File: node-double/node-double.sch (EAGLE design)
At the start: 33 parts, among them IC1 TP4056, IC3 24C02, U1 ATMEGA328P_TQFP, U2 3.3V/150mA

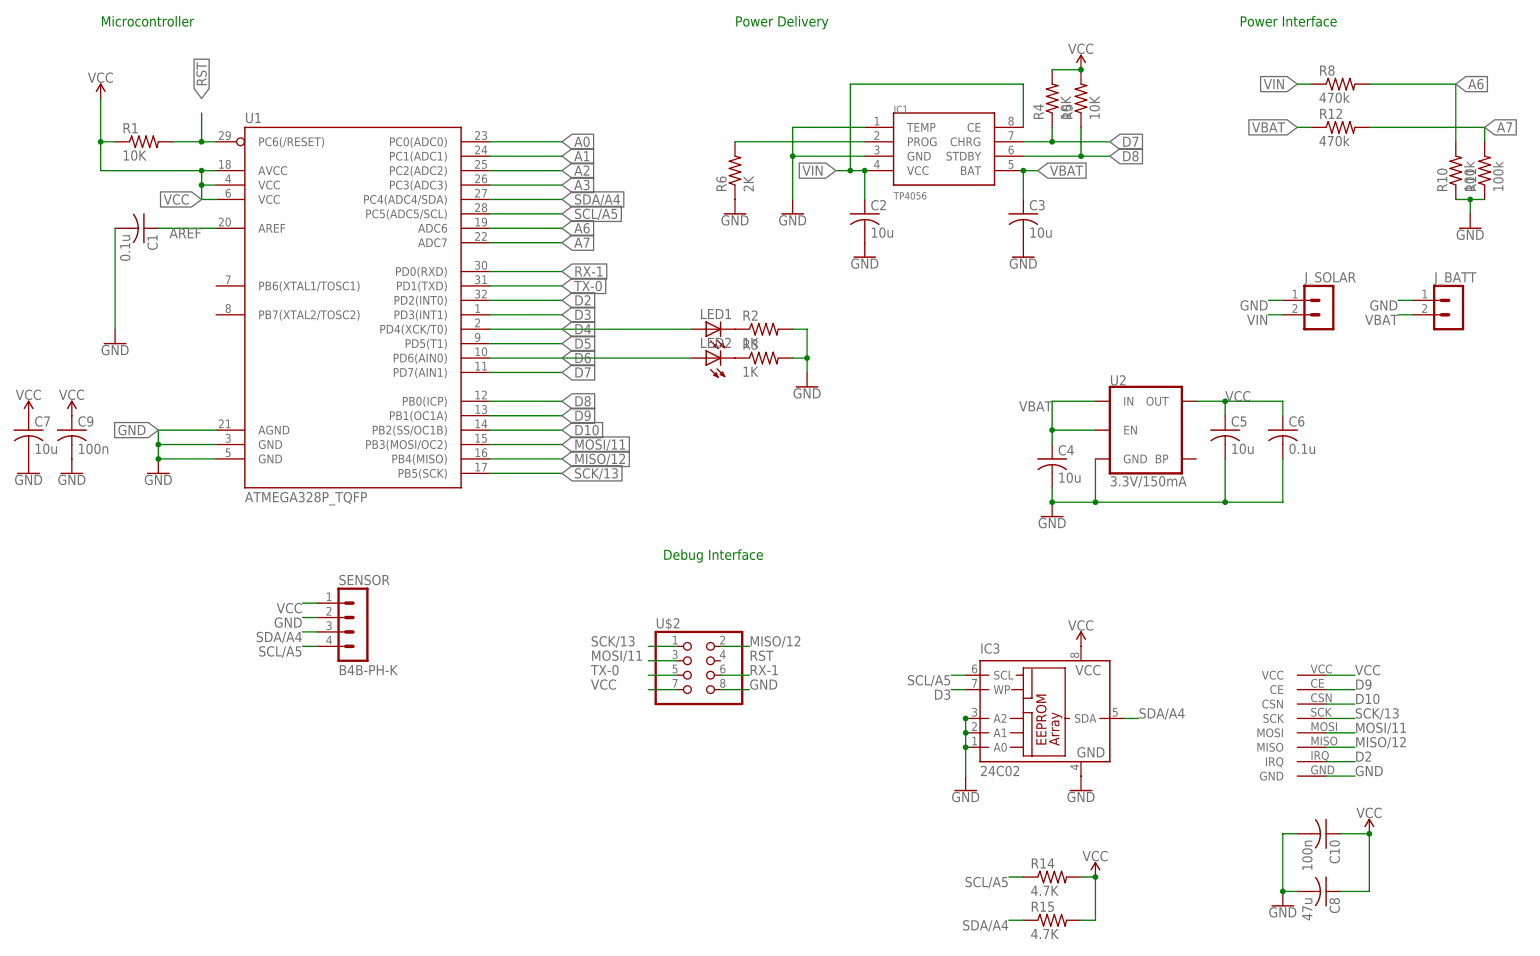
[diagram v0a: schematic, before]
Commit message: Scratch progress
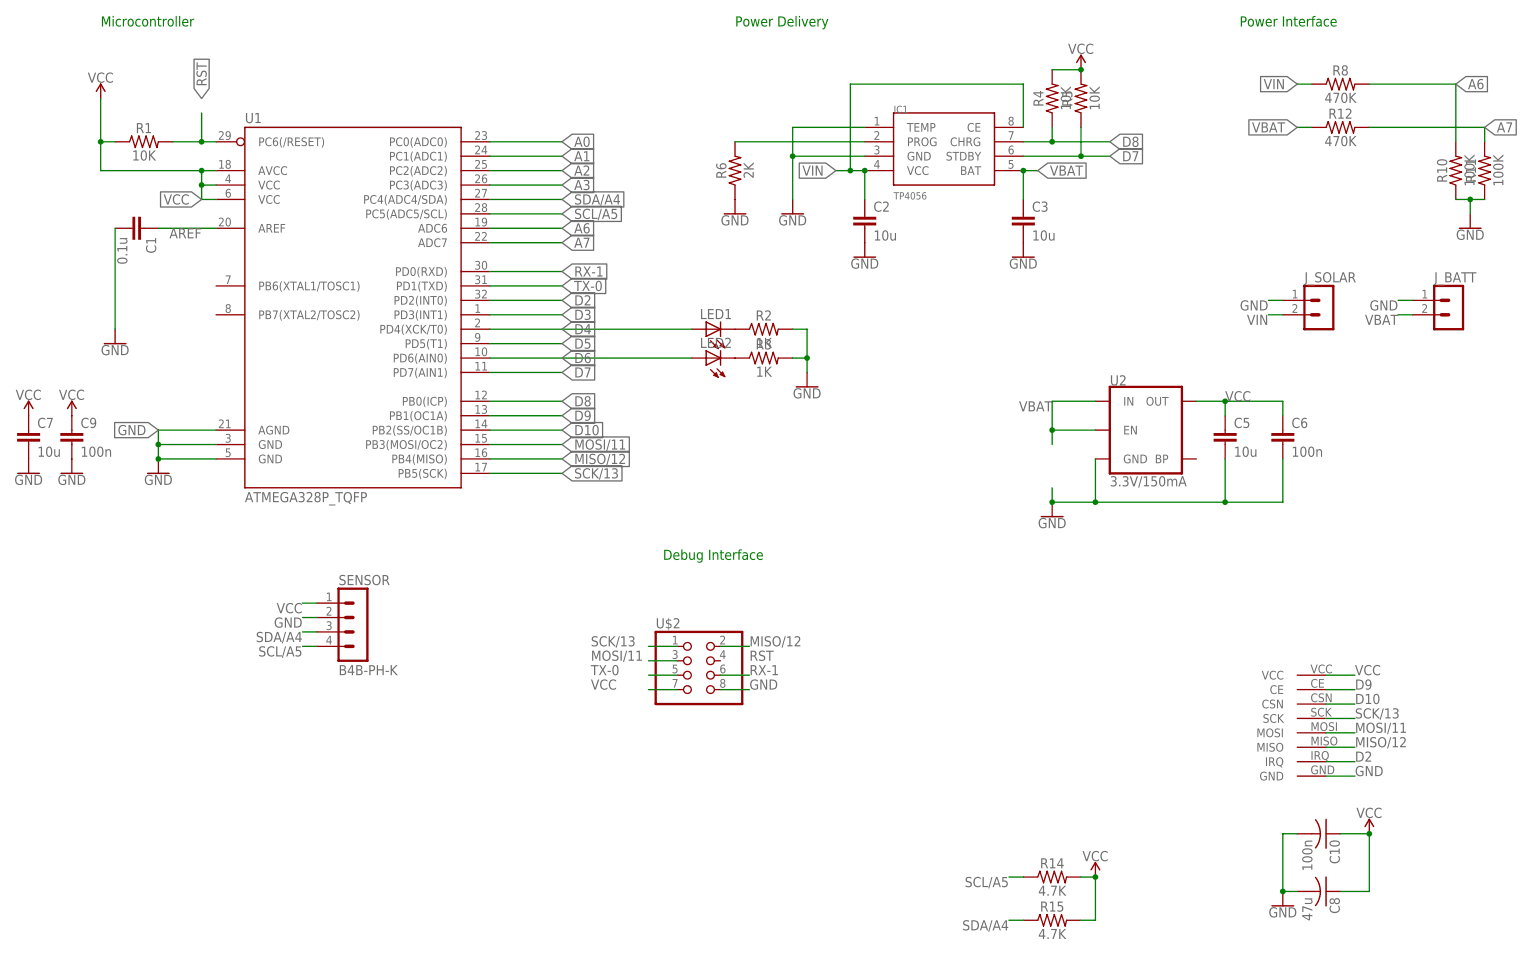
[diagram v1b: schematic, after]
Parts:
- removed C4: 10u, resistor:C-USC0603
- removed IC3: 24C02, microchip:24C02ASN
- C1, C2, C3, C5, C7, C9: device resistor:C-USC0603 -> Nordic_nRF:CAPACITOR_0603_L
- C6: value 0.1u -> 100n; device resistor:C-USC0603 -> Nordic_nRF:CAPACITOR_0603_L
- R1, R14, R15, R2, R3, R4, R5, R6: device resistor:R-US_R0603 -> SparkFun-Resistors:RESISTOR0603
- R10, R11: value 100k -> 100K; device resistor:R-US_R0603 -> SparkFun-Resistors:RESISTOR0603
- R12, R8: value 470k -> 470K; device resistor:R-US_R0603 -> SparkFun-Resistors:RESISTOR0603
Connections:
- net D3: no longer IC3.WP
- net D7: now also IC1.STDBY, R5.1; no longer IC1.CHRG, R4.1
- net D8: now also IC1.CHRG, R4.1; no longer IC1.STDBY, R5.1
- net GND: no longer C4.2, IC3.A0, IC3.A1, IC3.A2, IC3.GND
- net SCL/A5: no longer IC3.SCL
- net SDA/A4: no longer IC3.SDA
- net VBAT: no longer C4.1
- net VCC: no longer IC3.VCC
